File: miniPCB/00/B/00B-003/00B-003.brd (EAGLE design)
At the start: 28 parts, among them Q1 2N7002, U1 INA290

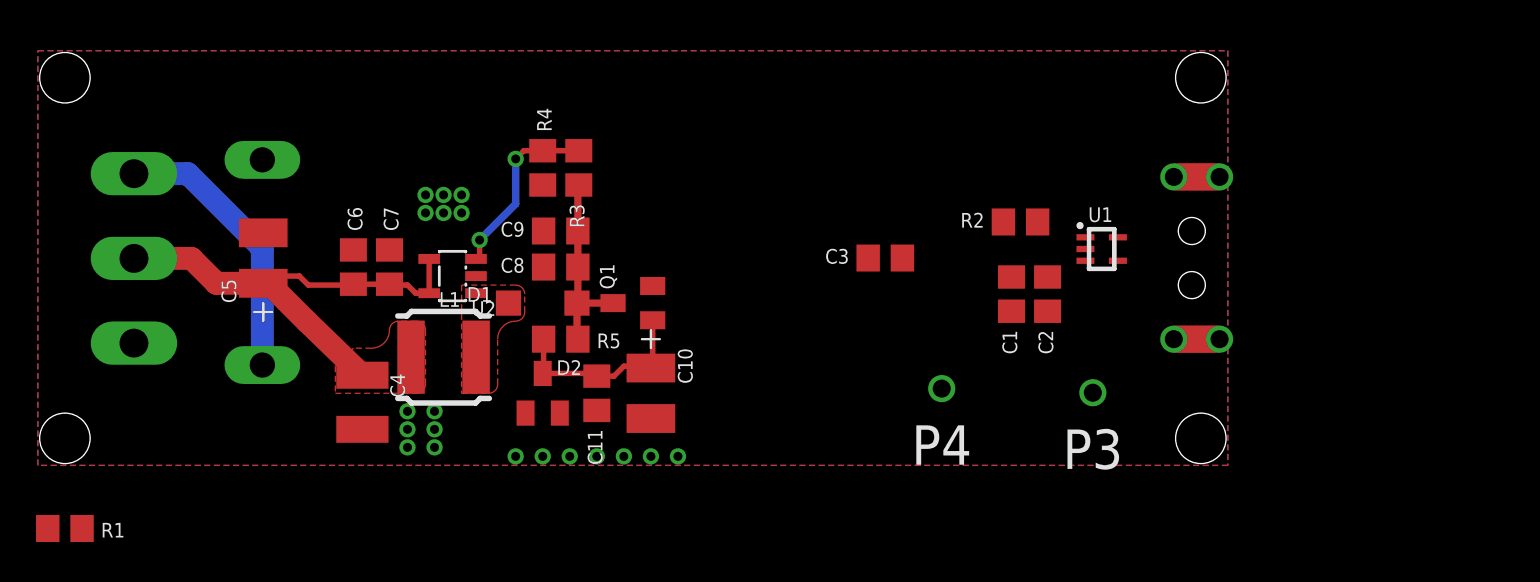
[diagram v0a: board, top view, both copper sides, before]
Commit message: NM.23OCT2023
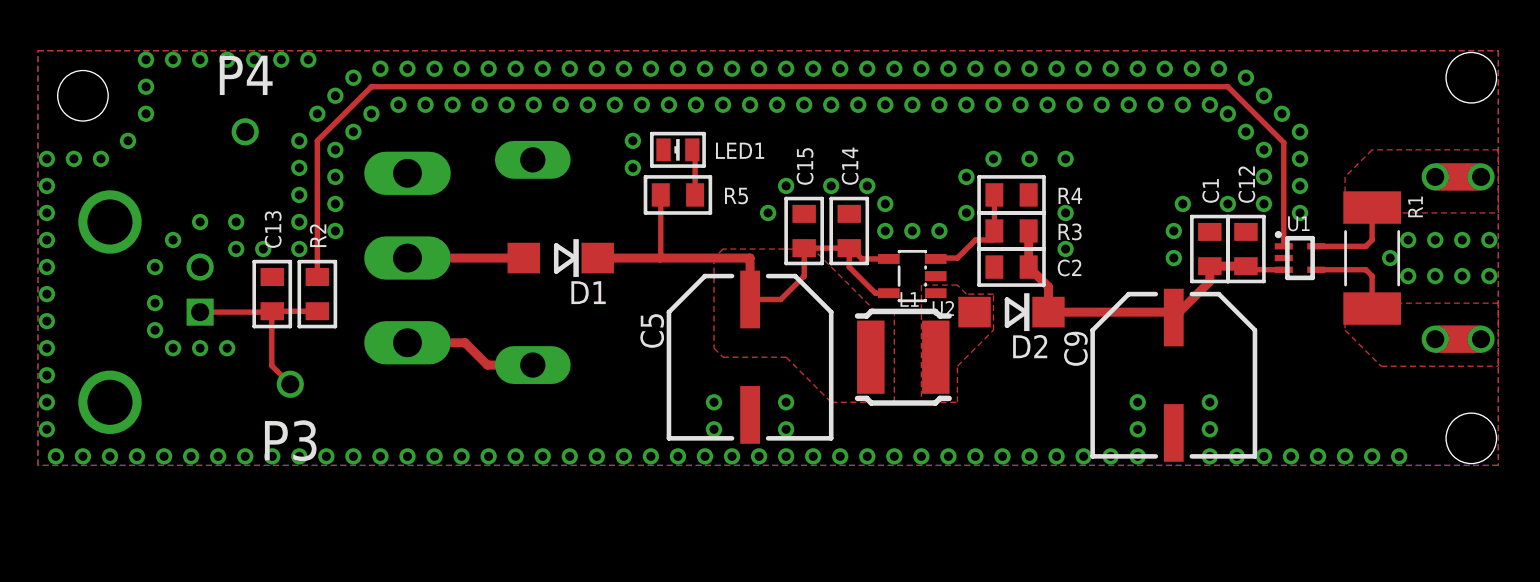
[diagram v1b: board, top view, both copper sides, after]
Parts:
- removed C10: 22u, nolan-utsa:C1210
- removed C11, C3, C7: 1n, nolan-utsa:C0805
- removed C4: 22u, nolan-utsa:C1210K
- removed C6, C8: 1u, nolan-utsa:C0805
- removed Q1: 2N7002, nolan-utsa:SOT23
- added C12, C14: 100n, minipcb:C0805
- added C13: 1n, minipcb:C0805
- added C15: 1u, minipcb:C0805
- added J1: (no value), minipcb:BNC_RIGHTANGLE
- added LED1: GREEN, minipcb:CHIP-LED0805
- C1: device nolan-utsa:C0805 -> minipcb:C0805
- C2: value 1n -> 100p; device nolan-utsa:C0805 -> minipcb:C0805
- C5: device nolan-utsa:C1210 -> nolan-utsa:C-PCR-8X10
- C9: device nolan-utsa:C0805 -> nolan-utsa:C-PCR-8X10
- D1: device nolan-utsa:SOD123-K -> minipcb:DO214AC
- D2: value 18V -> 1N5819; device nolan-utsa:SOT23 -> minipcb:DO214AC
- R1: device nolan-utsa:R0805 -> minipcb:R2512K
- R2: value 270 -> 250; device nolan-utsa:R0805 -> minipcb:R0805
- R3: value (none) -> 22000; device nolan-utsa:R0805 -> minipcb:R0805
- R4: value (none) -> 1200; device nolan-utsa:R0805 -> minipcb:R0805
- R5: value 10k -> 250; device nolan-utsa:R0805 -> minipcb:R0805
- U2: value (none) -> AP3012
- moved R1 74.0 mm to (75.0, 12.5), turned to 270 degrees
- moved P3 44.5 mm to (15.0, 5.50)
- moved P4 41.2 mm to (12.5, 19.5), turned to 0 degrees
- moved R2 39.2 mm to (16.5, 10.5), turned to 270 degrees
- moved C9 34.9 mm to (64.0, 6.00), turned to 0 degrees
- moved C5 27.6 mm to (40.5, 7.00), turned to 0 degrees
- moved D2 26.4 mm to (55.0, 9.50), turned to 180 degrees
- moved R4 26.0 mm to (55.0, 16.0), turned to 180 degrees
- moved L1 25.5 mm to (49.0, 7.00)
- moved U2 25.5 mm to (49.5, 11.5)
- moved R3 24.3 mm to (55.0, 14.0), turned to 0 degrees
- moved SW1 15.2 mm to (21.5, 12.5), turned to 180 degrees
- moved B1 15.0 mm to (26.0, 0.00)
- moved P1 14.5 mm to (78.5, 8.00)
- moved P2 14.5 mm to (78.5, 17.0)
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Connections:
- net N$1 renamed P
- net N$2 renamed N
- net N$3 renamed OUTSIGNAL
- removed net HV_DCDC: C8.1, C9.1, D1.C, Q1.3, R3.2, R5.2
- removed net N$13: C10.+, C11.1, D2.3, Q1.1, R5.1
- new net BSW: D1.A, SW1.2
- new net N$1: LED1.A, R5.1
- net B+: now also C14.1ASD, C15.1ASD, D1.C, R5.2; no longer C4.1, C6.1, C7.1, SW1.2
- net GND: now also C1.2ASDF, C12.2ASDF, C13.2ASDF, C14.2ASDF, C15.2ASDF, C2.2ASDF, C9.-, J1.2, LED1.C; no longer C1.2, C10.-, C11.2, C2.2, C3.2, C4.2, C6.2, C7.2, C8.2, C9.2, D2.1
- net HV: now also C1.1ASD, C12.1ASD, C2.1ASD, C9.+, D2.C, R3.2; no longer C1.1, C2.1, Q1.2
- net HV_SW: now also D2.A; no longer D1.A
- net SIGNAL: now also C13.1ASD, J1.1; no longer C3.1
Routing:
- net OUTSIGNAL: track 0.00 -> 69.4 mm
- net HV: track 0.00 -> 19.9 mm
- net SIGNAL: track 0.00 -> 11.0 mm
- net N$13: track 10.9 -> 0.00 mm
- net HV_DCDC: track 10.6 -> 0.00 mm
- net N$7: track 15.3 -> 7.46 mm
- net BSW: track 0.00 -> 6.45 mm
- net P: track 0.00 -> 5.04 mm
- net N: track 0.00 -> 5.04 mm
- net HV_FB: track 10.1 -> 6.23 mm, vias 2 -> 0
- net N$1: track 0.00 -> 2.56 mm
- net B+: track 27.0 -> 28.2 mm
- added copper zone on layer 1, net N
- added copper zone on layer 1, net P

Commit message: NM.08NOV2023
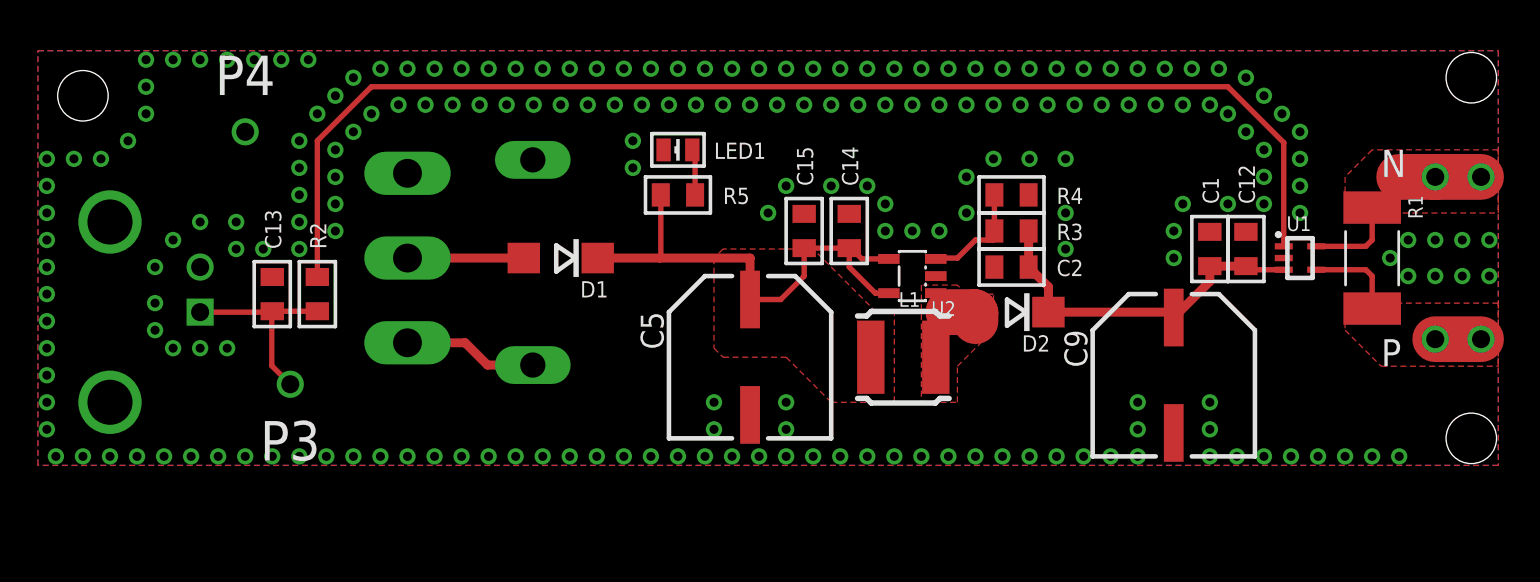
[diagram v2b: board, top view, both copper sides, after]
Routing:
- net N: track 5.04 -> 9.58 mm
- net P: track 5.04 -> 7.58 mm
- net HV_SW: track 0.00 -> 1.97 mm
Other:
- board text added: "B1"
- board text added: "C1"
- board text added: "C12"
- board text added: "C13"
- board text added: "C14"
- board text added: "C15"
- board text added: "C2"
- board text added: "C5"
- board text added: "C9"
- board text added: "D1"
- board text added: "D2"
- board text added: "J1"
- board text added: "L1"
- board text added: "LED1"
- board text added: "N"
- board text added: "P"
- board text added: "P3"
- board text added: "P4"
- board text added: "R1"
- board text added: "R2"
- board text added: "R3"
- board text added: "R4"
- board text added: "R5"
- board text added: "U1"
- board text added: "U2"
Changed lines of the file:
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@@
 <layer number="123" name="tTestmark" color="7" fill="1" visible="yes" active="yes"/>
 <layer number="124" name="bTestmark" color="7" fill="1" visible="yes" active="yes"/>
-<layer number="125" name="_tNames" color="7" fill="1" visible="yes" active="yes"/>
-<layer number="126" name="_bNames" color="7" fill="1" visible="yes" active="yes"/>
+<layer number="125" name="_tNames" color="14" fill="1" visible="yes" active="yes"/>
+<layer number="126" name="_bNames" color="5" fill="1" visible="yes" active="yes"/>
 <layer number="127" name="_tValues" color="7" fill="1" visible="yes" active="yes"/>
 <layer number="128" name="_bValues" color="7" fill="1" visible="yes" active="yes"/>
@@
 <wire x1="48.5" y1="4.5" x2="52.5" y2="4.5" width="0.5" layer="41"/>
 <wire x1="52.5" y1="4.5" x2="56" y2="8" width="0.5" layer="41"/>
-<wire x1="56" y1="8" x2="56" y2="10.5" width="0.5" layer="41"/>
-<wire x1="56" y1="10.5" x2="52.5" y2="10.5" width="0.5" layer="41"/>
-<wire x1="52.5" y1="10.5" x2="52" y2="11" width="0.5" layer="41"/>
-<wire x1="52" y1="11" x2="47.5" y2="11" width="0.5" layer="41"/>
+<wire x1="56" y1="8" x2="56" y2="11" width="0.5" layer="41"/>
+<wire x1="56" y1="11" x2="47.5" y2="11" width="0.5" layer="41"/>
 <wire x1="82" y1="19" x2="75" y2="19" width="0.3" layer="41"/>
 <wire x1="75" y1="19" x2="73" y2="17" width="0.3" layer="41"/>
@@
 <wire x1="73" y1="10.5" x2="82" y2="10.5" width="0.3" layer="42"/>
 <wire x1="55" y1="15" x2="55" y2="11" width="0.3" layer="41"/>
+<text x="75.5" y="6.5" size="1.5" layer="21" font="vector" ratio="12">P</text>
+<text x="75.5" y="17" size="1.5" layer="21" font="vector" ratio="12">N</text>
+<text x="26.499996875" y="24.000003125" size="1.27" layer="126" font="vector" rot="MR180">B1</text>
+<text x="66.49999375" y="15.49999375" size="0.899996875" layer="125" font="vector" ratio="13" rot="R90">C1</text>
+<text x="57.5000125" y="11.500003125" size="0.899996875" layer="125" font="vector" ratio="13">C2</text>
+<text x="35.706" y="9.524009375" size="1.27" layer="125" font="vector" ratio="12" rot="R270" align="top-left">C5</text>
+<text x="59.206003125" y="8.5240125" size="1.27" layer="125" font="vector" ratio="12" rot="R270" align="top-left">C9</text>
+<text x="68.499990625" y="15.49999375" size="0.899996875" layer="125" font="vector" ratio="13" rot="R90">C12</text>
+<text x="14.499996875" y="13" size="0.899996875" layer="125" font="vector" ratio="13" rot="R90">C13</text>
+<text x="46.500009375" y="16.49999375" size="0.899996875" layer="125" font="vector" ratio="13" rot="R90">C14</text>
+<text x="43.9999875" y="16.49999375" size="0.899996875" layer="125" font="vector" ratio="13" rot="R90">C15</text>
+<text x="32.639990625" y="11.213996875" size="0.899996875" layer="125" font="vector" ratio="10" rot="R180">D1</text>
+<text x="57.13999375" y="8.214003125" size="0.899996875" layer="125" font="vector" ratio="10" rot="R180">D2</text>
+<text x="12" y="2.49999375" size="1.499996875" layer="126" font="vector" ratio="12" rot="MR90">J1</text>
+<text x="48.746003125" y="9.7940125" size="0.8128" layer="125" font="vector">L1</text>
+<text x="38.5" y="17.999990625" size="0.899996875" layer="125" font="vector" ratio="12">LED1</text>
+<text x="14.999996875" y="3.4599875" size="2.1844" layer="125" font="vector" ratio="12" rot="R180" align="bottom-center">P3</text>
+<text x="12.5" y="21.5399875" size="2.1844" layer="125" font="vector" ratio="12" align="bottom-center">P4</text>
+<text x="76.999996875" y="15.99999375" size="0.8128" layer="125" font="vector" ratio="12" rot="R270">R1</text>
+<text x="16.999990625" y="13" size="0.899996875" layer="125" font="vector" ratio="13" rot="R90">R2</text>
+<text x="57.5000125" y="13.499996875" size="0.899996875" layer="125" font="vector" ratio="13">R3</text>
+<text x="57.5000125" y="15.49999375" size="0.899996875" layer="125" font="vector" ratio="13">R4</text>
+<text x="38.999996875" y="15.49999375" size="0.899996875" layer="125" font="vector" ratio="13">R5</text>
+<text x="70.25" y="13.999996875" size="0.8128" layer="125" font="vector" ratio="12">U1</text>
+<text x="51.913003125" y="10.103003125" size="0.8128" layer="125" font="vector" rot="R180">U2</text>
 </plain>
 <attributes>
@@
 <element name="U1" library="nolan-utsa" package="SC70-5" value="INA290" x="71" y="12.5" smashed="yes" rot="R270">
 <attribute name="NAME" x="70.25" y="14" size="0.8128" layer="25" font="vector" ratio="12"/>
-<attribute name="VALUE" x="71" y="10.5" size="0.8128" layer="27" font="vector" ratio="12" align="center"/>
 </element>
 <element name="P1" library="nolan-utsa" package="PINS_1_1MM" value="" x="78.5" y="8" smashed="yes"/>
@@
 </element>
 <element name="D2" library="minipcb" package="DO214AC" value="1N5819" x="55" y="9.5" smashed="yes" rot="R180">
-<attribute name="NAME" x="57.14" y="8.214" size="1.27" layer="25" font="vector" ratio="10" rot="R180"/>
-<attribute name="VALUE" x="57.64" y="12.056" size="1.27" layer="27" ratio="10" rot="R180"/>
+<attribute name="NAME" x="57.14" y="8.214" size="0.9" layer="25" font="vector" ratio="10" rot="R180"/>
 </element>
 <element name="D1" library="minipcb" package="DO214AC" value="1N5819" x="30" y="12.5" smashed="yes" rot="R180">
-<attribute name="NAME" x="32.64" y="11.214" size="1.27" layer="25" ratio="10" rot="R180"/>
-<attribute name="VALUE" x="32.64" y="15.056" size="1.27" layer="27" ratio="10" rot="R180"/>
+<attribute name="NAME" x="32.64" y="11.214" size="0.9" layer="25" font="vector" ratio="10" rot="R180"/>
 </element>
 <element name="J1" library="minipcb" package="BNC_RIGHTANGLE" value="" x="10" y="9.5" smashed="yes" rot="MR270">
@@
 <element name="R1" library="minipcb" package="R2512K" value="0R5" x="75" y="12.5" smashed="yes" rot="R270">
 <attribute name="NAME" x="77" y="16" size="0.8128" layer="25" font="vector" ratio="12" rot="R270"/>
-<attribute name="VALUE" x="73" y="9" size="0.8128" layer="27" font="vector" ratio="12" rot="R90"/>
 </element>
 <element name="C1" library="minipcb" package="C0805" value="1u" x="66" y="13" smashed="yes" rot="R90">
@@
 <contactref element="R1" pad="2"/>
 <wire x1="75" y1="9.7" x2="75" y2="11.5" width="0.3" layer="1"/>
+<wire x1="81.04" y1="8" x2="78.5" y2="8" width="2.54" layer="1"/>
 </signal>
 <signal name="N">
@@
 <contactref element="R1" pad="1"/>
 <wire x1="75" y1="13.5" x2="75" y2="15.3" width="0.3" layer="1"/>
-<wire x1="78.5" y1="17" x2="81.04" y2="17" width="0" layer="19" extent="1-1"/>
+<wire x1="78.5" y1="17" x2="76.5" y2="17" width="2.54" layer="1"/>
+<wire x1="81.04" y1="17" x2="78.5" y2="17" width="2.54" layer="1"/>
 </signal>
 <signal name="GND">
@@
 <vertex x="52" y="11"/>
 </polygon>
+<wire x1="52.95" y1="9.5" x2="51.5" y2="9.5" width="2.54" layer="1"/>
+<wire x1="52.95" y1="9.5" x2="53" y2="9.45" width="2.54" layer="1"/>
+<wire x1="53" y1="9.45" x2="53" y2="9" width="2.54" layer="1"/>
 </signal>
 <signal name="HV_FB">
